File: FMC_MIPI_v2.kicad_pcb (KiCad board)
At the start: 6 copper layers, 69.3 x 111.8 mm, 138 parts, among them IC1 SN74AVC4T245PWR, IC2 AT24MAC402-MAHM-T, IC3 TCA9406DCUR, IC4 TCA9406DCUR, IC5 TCA9406DCUR, IC6 SN74AVC1T45DCKT, IC7 SN74AVC1T45DCKT, J1 ASP-134488-01, J2 QTH-060-01-L-D-A, U1 LP5907MFX-1.8, U2 SN74AVC2T45DCUR, U3 SN74AVCH16T245_DGV_48, U4 TLV75525PDBV, U5 TS3DDR3812_RUA_42, U6 TS3DDR3812_RUA_42, U7 LP5907MFX-1.2, U8 SN74AVCH16T245_DGV_48

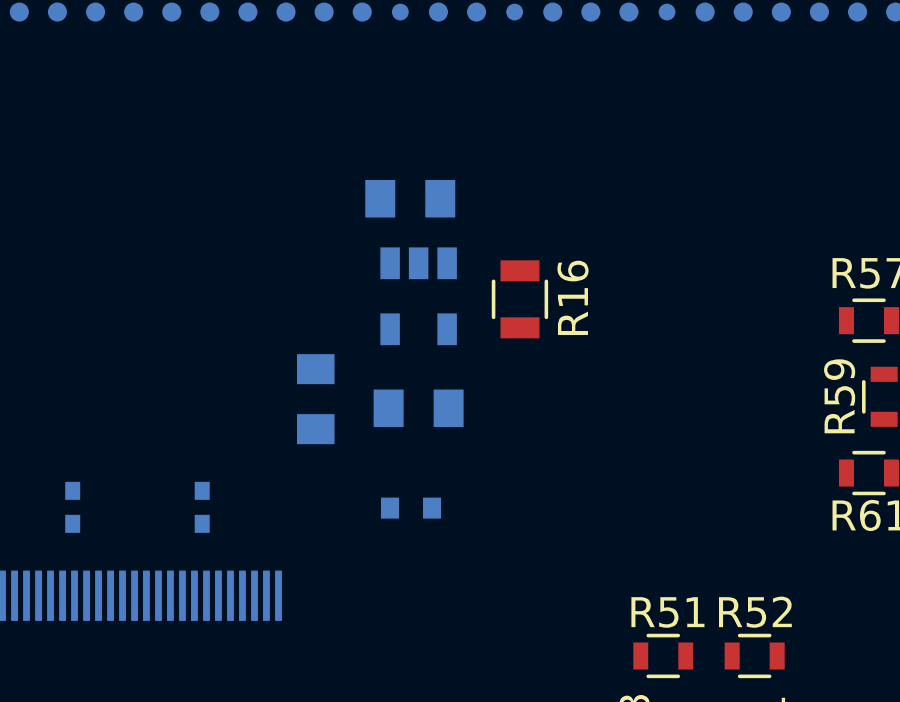
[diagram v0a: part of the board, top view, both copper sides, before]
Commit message: good, before FMC lines connect
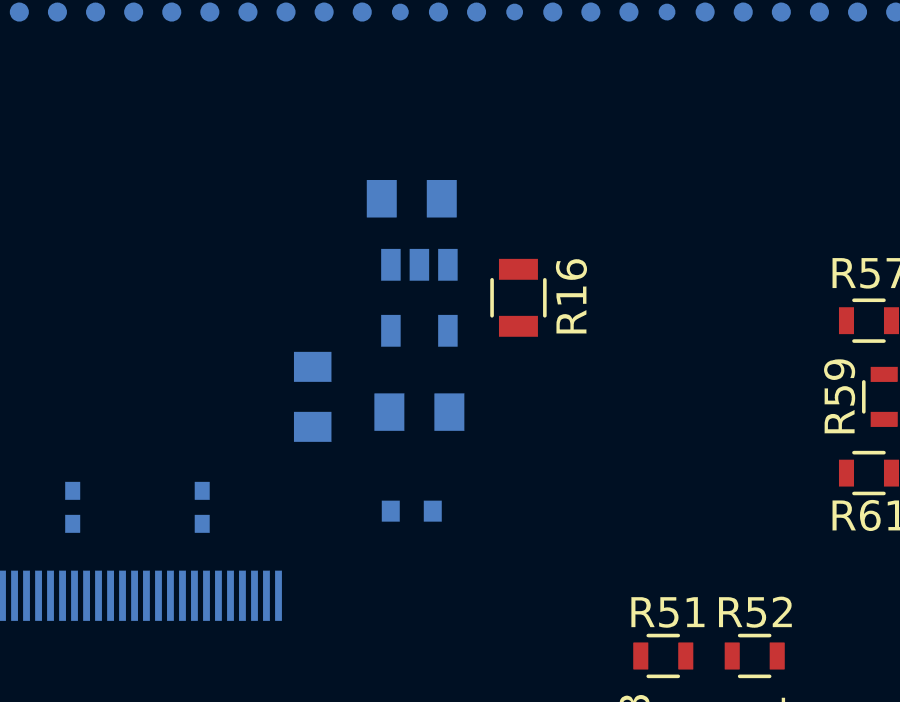
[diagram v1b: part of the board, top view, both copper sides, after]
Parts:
- moved C26 0.13 mm to (128.8, 58.9)
- moved C31 0.13 mm to (125.2, 58.4)
- moved D4 0.10 mm to (128.5, 62.2)
- moved R16 0.07 mm to (132.1, 55.1)
- moved U4 0.06 mm to (128.8, 55.1)
- moved C25 0.05 mm to (128.5, 51.8)
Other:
- net class Power added: clearance 0.1524, trace_width 0.254, via_dia 0.3556, via_drill 0.3048
- rule via_min_drill: 0.3 -> 0.127
- rule via_min_size: 0.4 -> 0.2032
